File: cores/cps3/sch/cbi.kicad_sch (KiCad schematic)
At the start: 1 part, among them K14 Am33C93A

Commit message: update6_cps
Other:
- company: (none) -> JOTEGO
- title: (none) -> CP SYSTEM III
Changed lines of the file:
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@@
 (kicad_sch (version 20211123) (generator eeschema)
   (paper "A4")
+  (title_block
+    (title "CP SYSTEM III")
+    (date "14/10/22")
+    (rev "José Tejada G.")
+    (company "JOTEGO")
+    (comment 1 "E.Triana")
+  )
   (junction (at 137.16 125.73) (diameter 0) (color 0 0 0 0)
   )

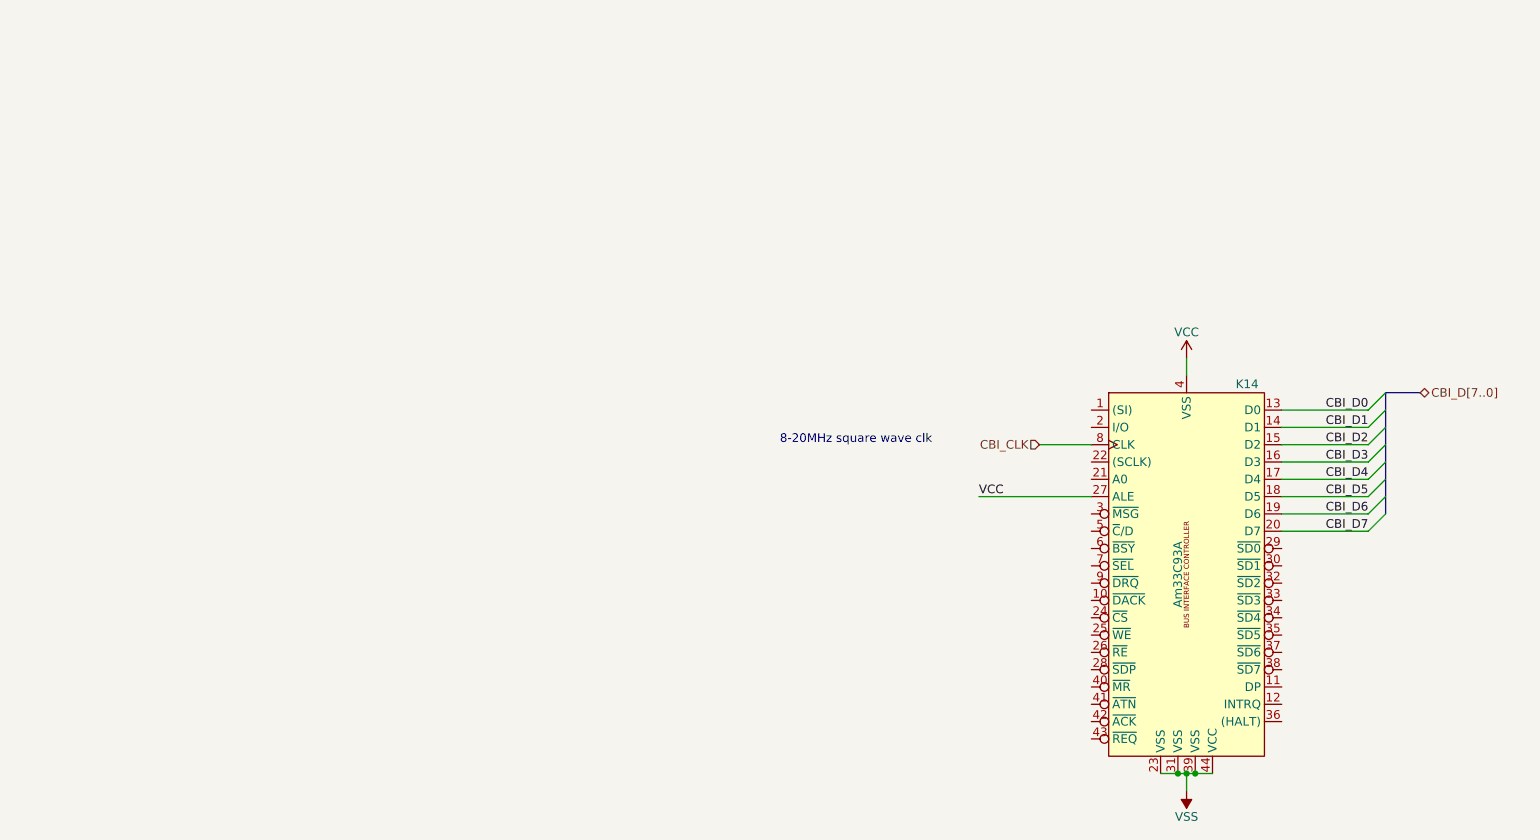
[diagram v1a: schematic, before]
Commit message: snd_colmix
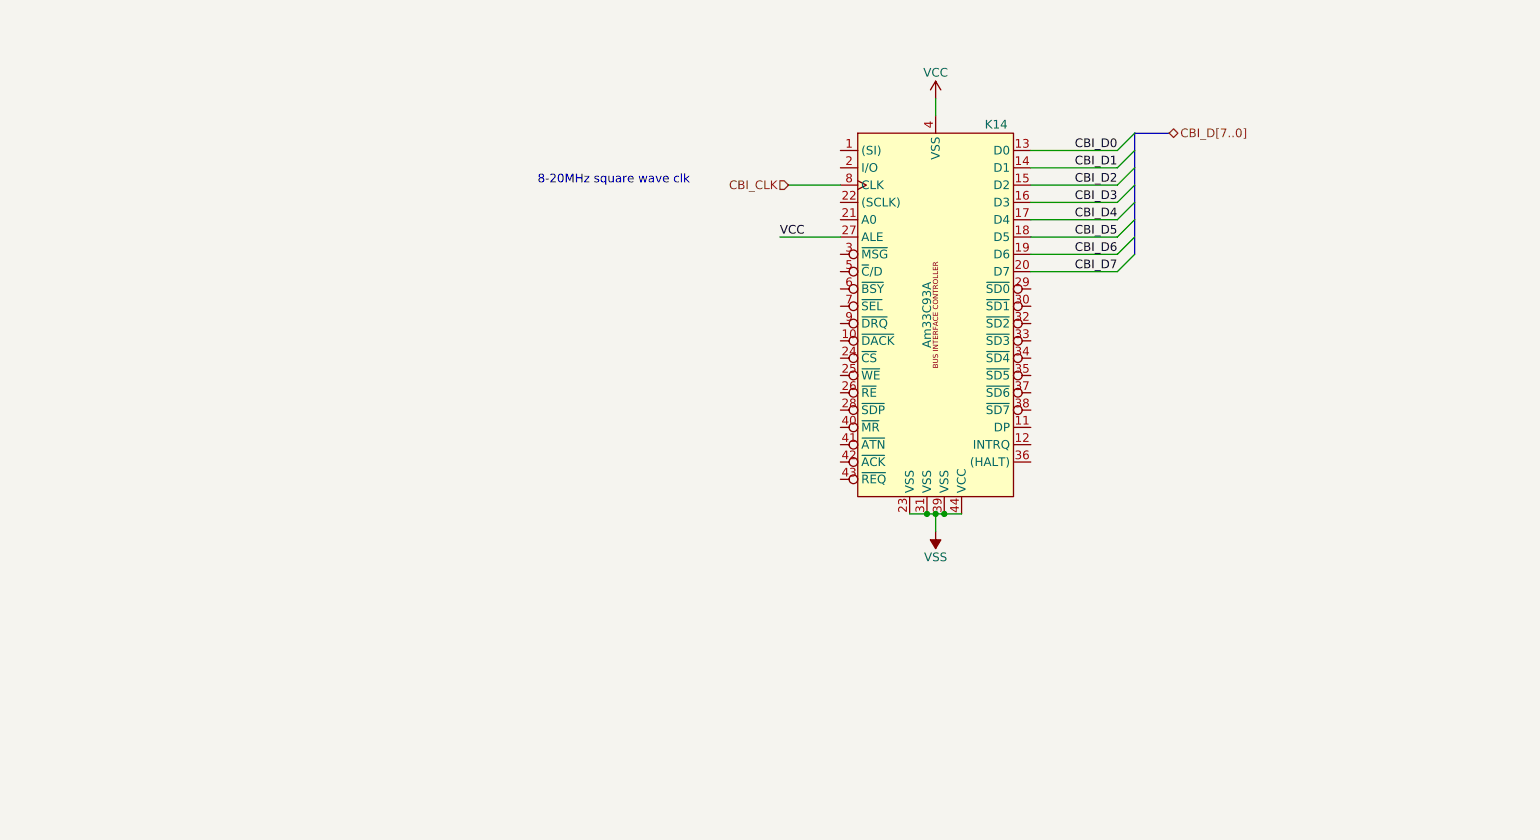
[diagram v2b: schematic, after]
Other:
- moved on the sheet: K14

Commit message: wip_cps3_vdac
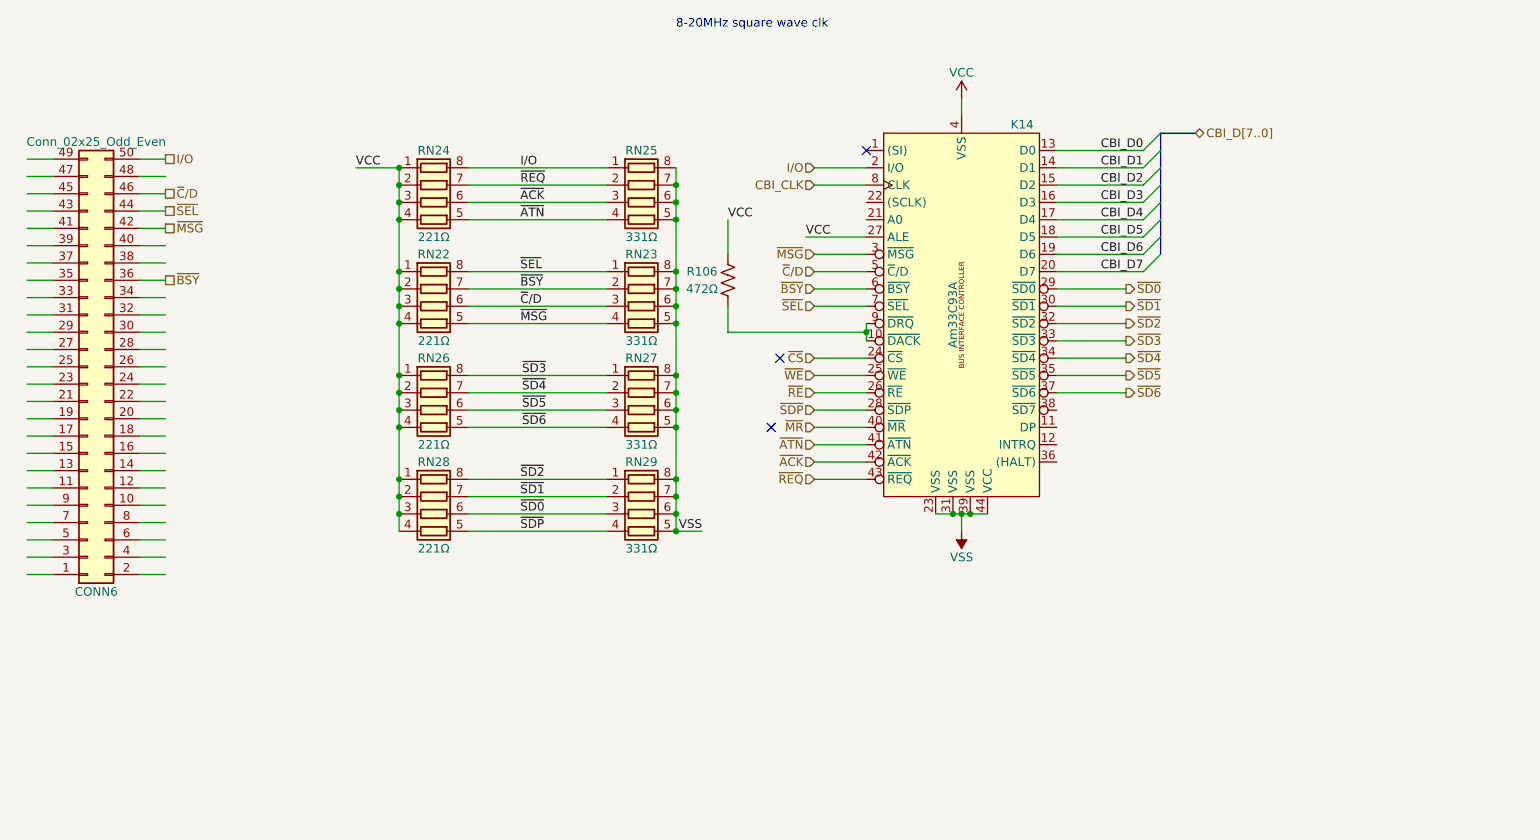
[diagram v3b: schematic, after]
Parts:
- added CONN6: Conn_02x25_Odd_Even, symbol Connector_Generic:Conn_02x25_Odd_Even
- added R106: 472Ω, symbol Device:R_US
- added RN22, RN24, RN26, RN28: 221Ω, symbol Device:R_Pack04
- added RN23, RN25, RN27, RN29: 331Ω, symbol Device:R_Pack04
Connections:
- net VCC: now also R106.1, RN22.1 (R1.1), RN22.2 (R2.1), RN22.3 (R3.1), RN22.4 (R4.1), RN24.1 (R1.1), RN24.2 (R2.1), RN24.3 (R3.1), RN24.4 (R4.1), RN26.1 (R1.1), RN26.2 (R2.1), RN26.3 (R3.1), RN26.4 (R4.1), RN28.1 (R1.1), RN28.2 (R2.1), RN28.3 (R3.1), RN28.4 (R4.1)
- net VSS: now also RN23.5 (R4.2), RN23.6 (R3.2), RN23.7 (R2.2), RN23.8 (R1.2), RN25.5 (R4.2), RN25.6 (R3.2), RN25.7 (R2.2), RN25.8 (R1.2), RN27.5 (R4.2), RN27.6 (R3.2), RN27.7 (R2.2), RN27.8 (R1.2), RN29.5 (R4.2), RN29.6 (R3.2), RN29.7 (R2.2), RN29.8 (R1.2)
- net at K14.10 (~{DACK}): now also K14.9 (~{DRQ}), R106.2
- net I/O: now reaches K14.2 (I/O)
- net I/O: now also CONN6.50 (Pin_50), RN24.8 (R1.2), RN25.1 (R1.1)
- net ~{CS}: now reaches K14.24 (~{CS})
- net ~{WE}: now reaches K14.25 (~{WE})
- net ~{RE}: now reaches K14.26 (~{RE})
- net ~{SDP}: now reaches K14.28 (~{SDP})
- net ~{SDP}: now also RN28.5 (R4.2), RN29.4 (R4.1)
- net ~{SD0}: now reaches K14.29 (~{SD0})
- net ~{SD0}: now also RN28.6 (R3.2), RN29.3 (R3.1)
- net ~{MSG}: now reaches K14.3 (~{MSG})
- net ~{MSG}: now also CONN6.42 (Pin_42), RN22.5 (R4.2), RN23.4 (R4.1)
- net ~{SD1}: now reaches K14.30 (~{SD1})
- net ~{SD1}: now also RN28.7 (R2.2), RN29.2 (R2.1)
- net ~{SD2}: now reaches K14.32 (~{SD2})
- net ~{SD2}: now also RN28.8 (R1.2), RN29.1 (R1.1)
- net ~{SD3}: now reaches K14.33 (~{SD3})
- net ~{SD3}: now also RN26.8 (R1.2), RN27.1 (R1.1)
- net ~{SD4}: now reaches K14.34 (~{SD4})
- net ~{SD4}: now also RN26.7 (R2.2), RN27.2 (R2.1)
- net ~{SD5}: now reaches K14.35 (~{SD5})
- net ~{SD5}: now also RN26.6 (R3.2), RN27.3 (R3.1)
- net ~{SD6}: now reaches K14.37 (~{SD6})
- net ~{SD6}: now also RN26.5 (R4.2), RN27.4 (R4.1)
- net ~{MR}: now reaches K14.40 (~{MR})
- net ~{ATN}: now reaches K14.41 (~{ATN})
- net ~{ATN}: now also RN24.5 (R4.2), RN25.4 (R4.1)
- net ~{ACK}: now reaches K14.42 (~{ACK})
- net ~{ACK}: now also RN24.6 (R3.2), RN25.3 (R3.1)
- net ~{REQ}: now reaches K14.43 (~{REQ})
- net ~{REQ}: now also RN24.7 (R2.2), RN25.2 (R2.1)
- net ~{C}/D: now reaches K14.5 (~{C}/D)
- net ~{C}/D: now also CONN6.46 (Pin_46), RN22.6 (R3.2), RN23.3 (R3.1)
- net ~{BSY}: now reaches K14.6 (~{BSY})
- net ~{BSY}: now also CONN6.36 (Pin_36), RN22.7 (R2.2), RN23.2 (R2.1)
- net ~{SEL}: now reaches K14.7 (~{SEL})
- net ~{SEL}: now also CONN6.44 (Pin_44), RN22.8 (R1.2), RN23.1 (R1.1)
- no-connect marks 0 -> 3
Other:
- moved on the sheet: K14
